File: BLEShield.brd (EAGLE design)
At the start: 25.4 x 39.4 mm, 34 parts, among them IC1 HEF4050BT, IC2 NRF8001, IC3 MCP1700T-3002E, J1 Debug/Test UART, J2 Interface, Q1 2N7002, Q2 16 MHz, Q3 32768 Hz

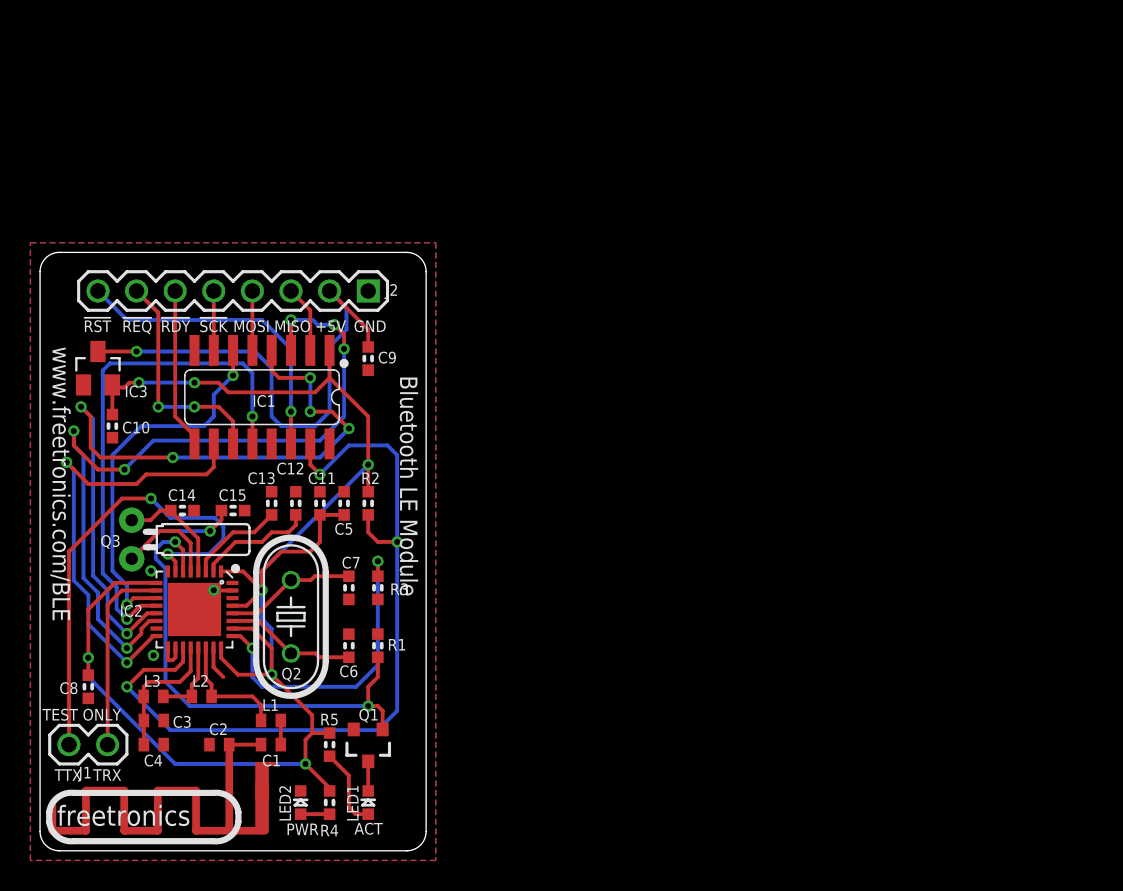
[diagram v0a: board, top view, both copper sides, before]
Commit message: checked files are the right ones
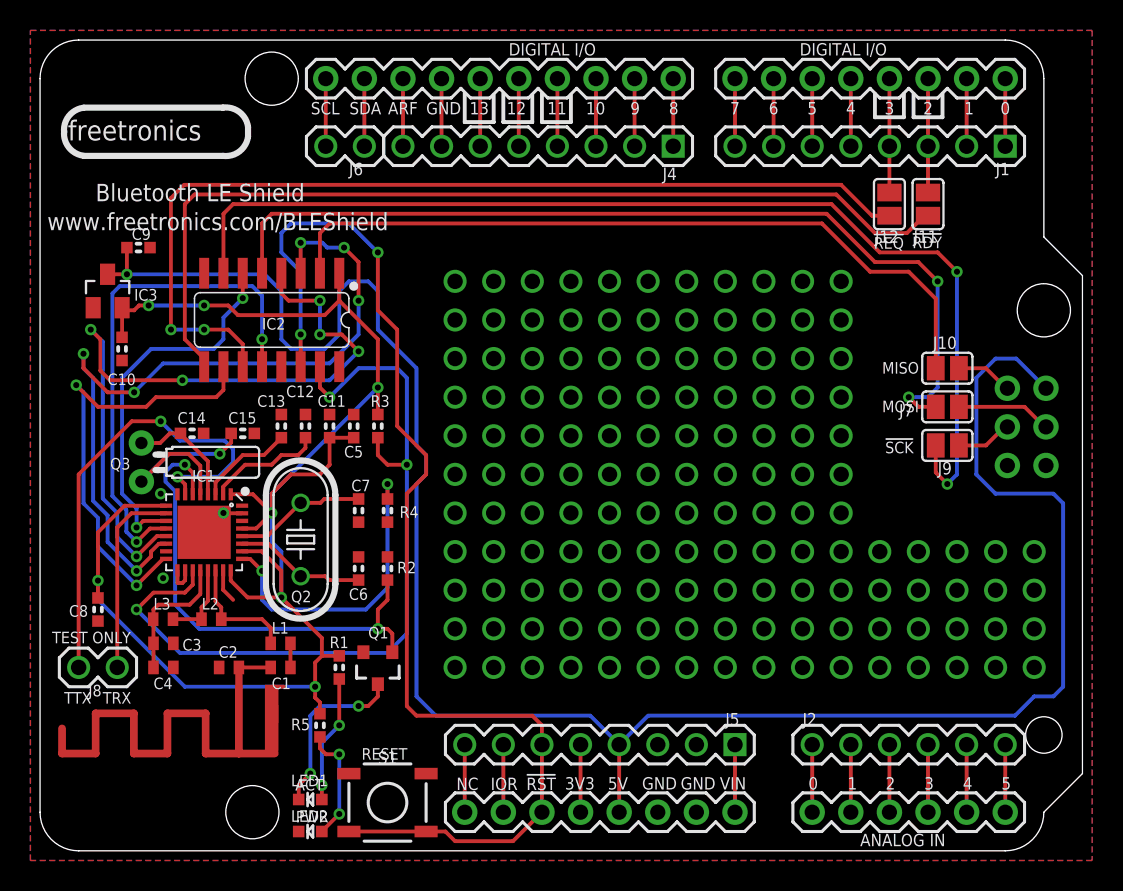
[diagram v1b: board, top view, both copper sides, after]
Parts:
- added J10, J11, J12, J7, J9: SJ, freetronics-luke:SJ
- added J3: ARDUINO-SHIELD_R3, freetronics-luke:ARDUINO-SHIELD_R3
- added J4, J5: (no value), freetronics-master-v1:1X08
- added J6: (no value), freetronics-master-v1:1X02
- added J8: Debug/Test UART, freetronics-master-v1:1X02
- added S1: Reset, freetronics:TACTILE_SWITCH_SMD
- IC1: value HEF4050BT -> NRF8001; device 40xx:SO16 -> bluetooth:FITNESSDEVICE_QFN-32
- IC2: value NRF8001 -> HEF4050BT; device bluetooth:FITNESSDEVICE_QFN-32 -> 40xx:SO16
- J1: value Debug/Test UART -> (none); device freetronics-master-v1:1X02 -> freetronics-master-v1:1X08
- J2: value Interface -> (none); device freetronics-master-v1:1X08 -> freetronics-master-v1:1X06
- R1: value 100kΩ -> 1kΩ
- R2: value 10kΩ -> 100kΩ
- R3: value 22kΩ 1% -> 10kΩ
- R4: value 1kΩ -> 22kΩ 1%
- moved J1 71.0 mm to (64.1, 47.0)
- moved J2 41.8 mm to (51.4, 7.62), turned to 0 degrees
- moved IC2 19.7 mm to (15.9, 35.6)
- moved R4 19.6 mm to (23.5, 23.0), turned to 270 degrees
- moved C9 16.8 mm to (7.11, 40.3), turned to 180 degrees
- moved R3 10.6 mm to (22.9, 28.6)
- moved IC1 9.67 mm to (11.4, 21.6)
- moved IC3 5.12 mm to (5.08, 37.5)
- moved C10 5.12 mm to (6.03, 33.7)
- moved C7 5.12 mm to (21.6, 23.0)
- moved C8 5.12 mm to (4.45, 16.5)
- moved Q3 5.12 mm to (7.30, 26.2)
- moved ANT1 5.12 mm to (15.9, 11.4)
- moved C3 5.12 mm to (8.75, 14.3)
- moved L1 5.12 mm to (16.5, 14.3)
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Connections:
- removed net !RDY_5V: IC1.9, J2.6
- removed net !REQ_5V: IC1.11, J2.7
- new net +3.3V: J3.3V3, J5.5
- new net A: IC2.5, J7.1
- new net A0: J2.1, J3.A0
- new net B: IC2.7, J9.1
- new net C: IC2.9, J11.1
- new net D: IC2.11, J12.1
- new net D2: J1.3, J11.2, J3.D2
- new net D3: J1.4, J12.2, J3.D3
- new net N$123: J1.6, J3.D5
- new net N$124: J1.7, J3.D6
- new net N$125: J1.8, J3.D7
- new net N$126: J3.SDA, J6.1
- new net N$127: J3.AREF, J4.8
- new net N$128: J3.D13, J4.6
- new net N$129: J3.D12, J4.5
- new net N$130: J3.SCL, J6.2
- new net N$131: J3.D8, J4.1
- new net N$132: J3.D9, J4.2
- new net N$133: J3.D10, J4.3
- new net N$134: J3.D11, J4.4
- new net N$18: IC2.2, J10.1
- new net N$27: J2.2, J3.A1
- new net N$37: J2.3, J3.A2
- new net N$50: J2.4, J3.A3
- new net N$72: J2.5, J3.A4
- new net N$73: J2.6, J3.A5
- new net N$74: J3.RESERVED, J5.8
- new net N$75: J3.VIN, J5.1
- new net N$81: J3.IOREF, J5.7
- new net N$82: J1.1, J3.D0
- new net N$87: J1.2, J3.D1
- new net N$90: J1.5, J3.D4
- net !RDY: now also IC1.16, IC2.10; no longer IC1.10, IC2.16
- net !RESET: now also IC1.19, IC2.15, R3.2; no longer IC1.15, IC2.19, R2.2
- net !RESET_5V: now also IC2.14, J3.!RESET, J5.6, S1.3, S1.4; no longer IC1.14, J2.8
- net +3.0V: now also IC1.24, IC1.26, IC1.29, IC1.9, R1.1, R3.1, R5.2; no longer IC2.24, IC2.26, IC2.29, IC2.9, R2.1, R4.2, R5.1
- net +5V: now also J3.+5V, J3.+5V@0, J5.4; no longer J2.2
- net ACTIVE: now also IC1.6, R2.1; no longer IC2.6, R1.1
- net ANT1: now also IC1.21; no longer IC2.21
- net ANT2: now also IC1.22; no longer IC2.22
- net GND: now also IC1.17, IC1.18, IC1.23, IC1.30, IC1.31, IC1.EP, J3.GND, J3.GND@0, J3.GND@1, J3.GND@2, J4.7, J5.2, J5.3, R2.2, R4.2, S1.1, S1.2; no longer IC2.17, IC2.18, IC2.23, IC2.30, IC2.31, IC2.EP, J2.1, R1.2, R3.2
- net MISO: now also IC1.14, IC2.3; no longer IC1.3, IC2.14
- net MISO_5V: now also J10.2, J3.MISO; no longer IC1.2, J2.3
- net MOSI: now also IC1.13, IC2.4; no longer IC1.4, IC2.13
- net MOSI_5V: now also J3.MOSI, J7.2; no longer IC1.5, J2.4
- net N$1: now also IC1.2; no longer IC2.2
- net N$14: now also R5.1; no longer R4.1
- net N$17: now also R1.2; no longer R5.2
- net N$2: now also IC1.3; no longer IC2.3
- net N$3: now also IC1.25, R4.1; no longer IC2.25, R3.1
- net N$4: now also IC1.28; no longer IC2.28
- net N$5: now also IC1.27; no longer IC2.27
- net N$6: now also IC1.4; no longer IC2.4
- net N$7: now also IC1.5; no longer IC2.5
- net RXD: now also IC1.10, J8.1; no longer IC2.10, J1.1
- net SCK: now also IC1.11, IC2.6; no longer IC1.6, IC2.11
- net SCK_5V: now also J3.SCK, J9.2; no longer IC1.7, J2.5
- net TXD: now also IC1.7, J8.2; no longer IC2.7, J1.2
- net VDD_PA: now also IC1.20; no longer IC2.20
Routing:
- net +5V: track 33.1 -> 136.2 mm
- net B: track 0.00 -> 71.4 mm, vias 0 -> 2
- net D: track 0.00 -> 63.7 mm, vias 0 -> 2
- net C: track 0.00 -> 61.9 mm
- net A: track 0.00 -> 61.0 mm, vias 0 -> 2
- net !RESET_5V: track 20.5 -> 77.3 mm, vias 1 -> 2
- net N$18: track 0.00 -> 50.0 mm
- net !REQ_5V: track 15.0 -> 0.00 mm, vias 2 -> 0
- net !RDY_5V: track 10.6 -> 0.00 mm
- net N$15: track 1.95 -> 11.6 mm, vias 0 -> 2
- net D3: track 0.00 -> 7.49 mm
- net D2: track 0.00 -> 7.49 mm
- net N$14: track 1.90 -> 7.73 mm, vias 0 -> 2
- net N$90: track 0.00 -> 4.45 mm
- net N$87: track 0.00 -> 4.45 mm
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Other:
- board size 25.4 x 39.4 mm -> 68.6 x 53.3 mm
- board text added: "Bluetooth LE Shield"
- board text added: "RESET"
- board text added: "www.freetronics.com/BLEShield"
- board text removed: "!RST"
- board text removed: "+5V"
- board text removed: "Bluetooth LE Module"
- board text removed: "GND"
- board text removed: "www.freetronics.com/BLE"
